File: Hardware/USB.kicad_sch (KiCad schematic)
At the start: 28 parts, among them Q1 MBT3904DW1, U3 CH340C, U9 USB251xB, Y1 24MHz

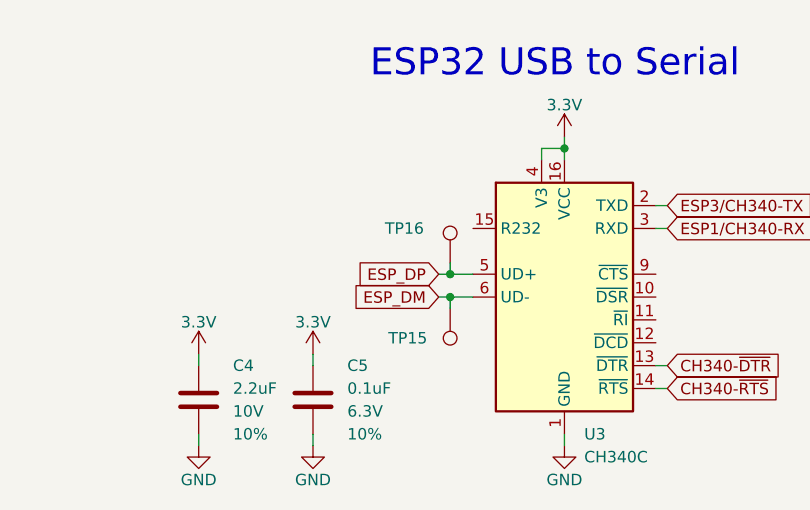
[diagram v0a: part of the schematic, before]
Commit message: Work in progress...
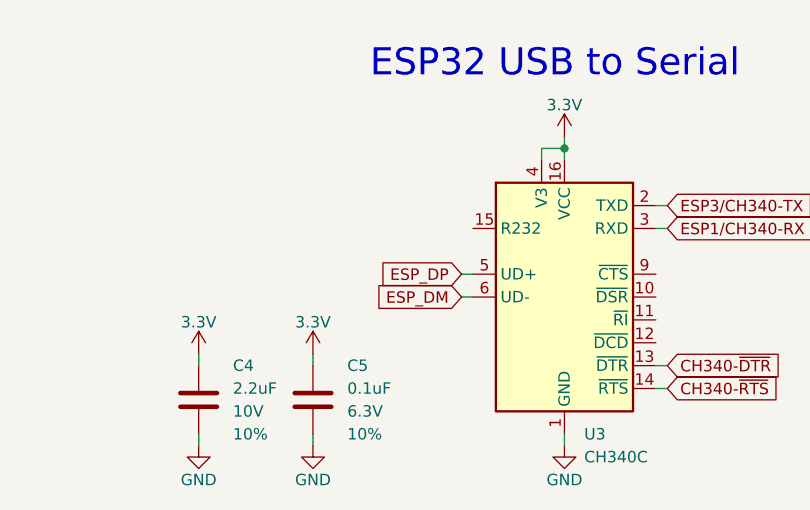
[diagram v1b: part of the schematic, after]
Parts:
- removed TP15, TP16: PTH, SparkFun-Connector:1X01, symbol SparkFun-Connector:TestPoint_PTH
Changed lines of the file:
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@@
   (junction (at 93.98 45.72) (diameter 0) (color 0 0 0 0)
   )
-  (junction (at 110.49 129.54) (diameter 0) (color 0 0 0 0)
-  )
   (junction (at 173.99 139.7) (diameter 0) (color 0 0 0 0)
   )
@@
   (junction (at 162.56 73.66) (diameter 0) (color 0 0 0 0)
   )
-  (junction (at 110.49 127) (diameter 0) (color 0 0 0 0)
-  )
   (junction (at 123.19 113.03) (diameter 0) (color 0 0 0 0)
   )
@@
     (stroke (width 0) (type default))
   )
-  (wire (pts (xy 110.49 125.73) (xy 110.49 127))
-    (stroke (width 0) (type default))
-  )
   (wire (pts (xy 182.88 38.1) (xy 116.84 38.1))
     (stroke (width 0) (type default))
@@
     (stroke (width 0) (type default))
   )
-  (wire (pts (xy 110.49 129.54) (xy 113.03 129.54))
-    (stroke (width 0) (type default))
-  )
   (wire (pts (xy 82.55 137.16) (xy 82.55 135.89))
     (stroke (width 0) (type default))
@@
     (stroke (width 0) (type default))
   )
-  (wire (pts (xy 109.22 127) (xy 110.49 127))
-    (stroke (width 0) (type default))
-  )
   (wire (pts (xy 181.61 78.74) (xy 181.61 80.01))
     (stroke (width 0) (type default))
@@
     (stroke (width 0) (type default))
   )
-  (wire (pts (xy 109.22 129.54) (xy 110.49 129.54))
+  (wire (pts (xy 111.76 129.54) (xy 113.03 129.54))
     (stroke (width 0) (type default))
   )
@@
     (stroke (width 0) (type default))
   )
-  (wire (pts (xy 110.49 129.54) (xy 110.49 130.81))
-    (stroke (width 0) (type default))
-  )
-  (wire (pts (xy 110.49 127) (xy 113.03 127))
+  (wire (pts (xy 111.76 127) (xy 113.03 127))
     (stroke (width 0) (type default))
   )
@@
     )
   )
-  (global_label "ESP_DM" (shape input) (at 109.22 129.54 180) (fields_autoplaced)
+  (global_label "ESP_DM" (shape input) (at 111.76 129.54 180) (fields_autoplaced)
     (effects (font (size 1.27 1.27)) (justify right))
-    (property "Intersheetrefs" "${INTERSHEET_REFS}" (at 98.9173 129.54 0)
+    (property "Intersheetrefs" "${INTERSHEET_REFS}" (at 101.4573 129.54 0)
       (effects (font (size 1.27 1.27)) (justify right) hide)
     )
   )
-  (global_label "ESP_DP" (shape input) (at 109.22 127 180) (fields_autoplaced)
+  (global_label "ESP_DP" (shape input) (at 111.76 127 180) (fields_autoplaced)
     (effects (font (size 1.27 1.27)) (justify right))
-    (property "Intersheetrefs" "${INTERSHEET_REFS}" (at 99.0987 127 0)
+    (property "Intersheetrefs" "${INTERSHEET_REFS}" (at 101.6387 127 0)
       (effects (font (size 1.27 1.27)) (justify right) hide)
     )
@@
         (path "/e3dd3ae4-244d-4cba-9cca-5d2abf83f29a/0cda3e5b-c4bb-4a16-94d7-679fa3b0b0b8"
           (reference "C5") (unit 1)
-        )
-      )
-    )
-  )
-  (symbol (lib_id "SparkFun-Connector:TestPoint_PTH") (at 110.49 130.81 180) (unit 1)
-    (in_bom yes) (on_board yes) (dnp no) (fields_autoplaced)
-    (property "Reference" "TP15" (at 107.95 134.112 0)
-      (effects (font (size 1.27 1.27)) (justify left))
-    )
-    (property "Value" "PTH" (at 110.49 127 0)
-      (effects (font (size 1.27 1.27)) hide)
-    )
-    (property "Footprint" "SparkFun-Connector:1X01" (at 111.76 124.46 0)
-      (effects (font (size 1.27 1.27)) hide)
-    )
-    (property "Datasheet" "~" (at 110.49 123.19 0)
-      (effects (font (size 1.27 1.27)) hide)
-    )
-    (pin "1")
-    (instances
-      (project "SparkFun_RTK_Facet_mosaic"
-        (path "/e3dd3ae4-244d-4cba-9cca-5d2abf83f29a/0cda3e5b-c4bb-4a16-94d7-679fa3b0b0b8"
-          (reference "TP15") (unit 1)
         )
       )
@@
         )
       )
-    )
-  )
-  (symbol (lib_id "SparkFun-Connector:TestPoint_PTH") (at 110.49 125.73 0) (unit 1)
-    (in_bom yes) (on_board yes) (dnp no)
-    (property "Reference" "TP16" (at 105.41 121.92 0)
-      (effects (font (size 1.27 1.27)))
-    )
-    (property "Value" "PTH" (at 110.49 129.54 0)
-      (effects (font (size 1.27 1.27)) hide)
-    )
-    (property "Footprint" "SparkFun-Connector:1X01" (at 109.22 132.08 0)
-      (effects (font (size 1.27 1.27)) hide)
-    )
-    (property "Datasheet" "~" (at 110.49 133.35 0)
-      (effects (font (size 1.27 1.27)) hide)
-    )
-    (pin "1")
-    (instances
-      (project "SparkFun_RTK_Facet_mosaic"
-        (path "/e3dd3ae4-244d-4cba-9cca-5d2abf83f29a/0cda3e5b-c4bb-4a16-94d7-679fa3b0b0b8"
-          (reference "TP16") (unit 1)
-        )
-      )

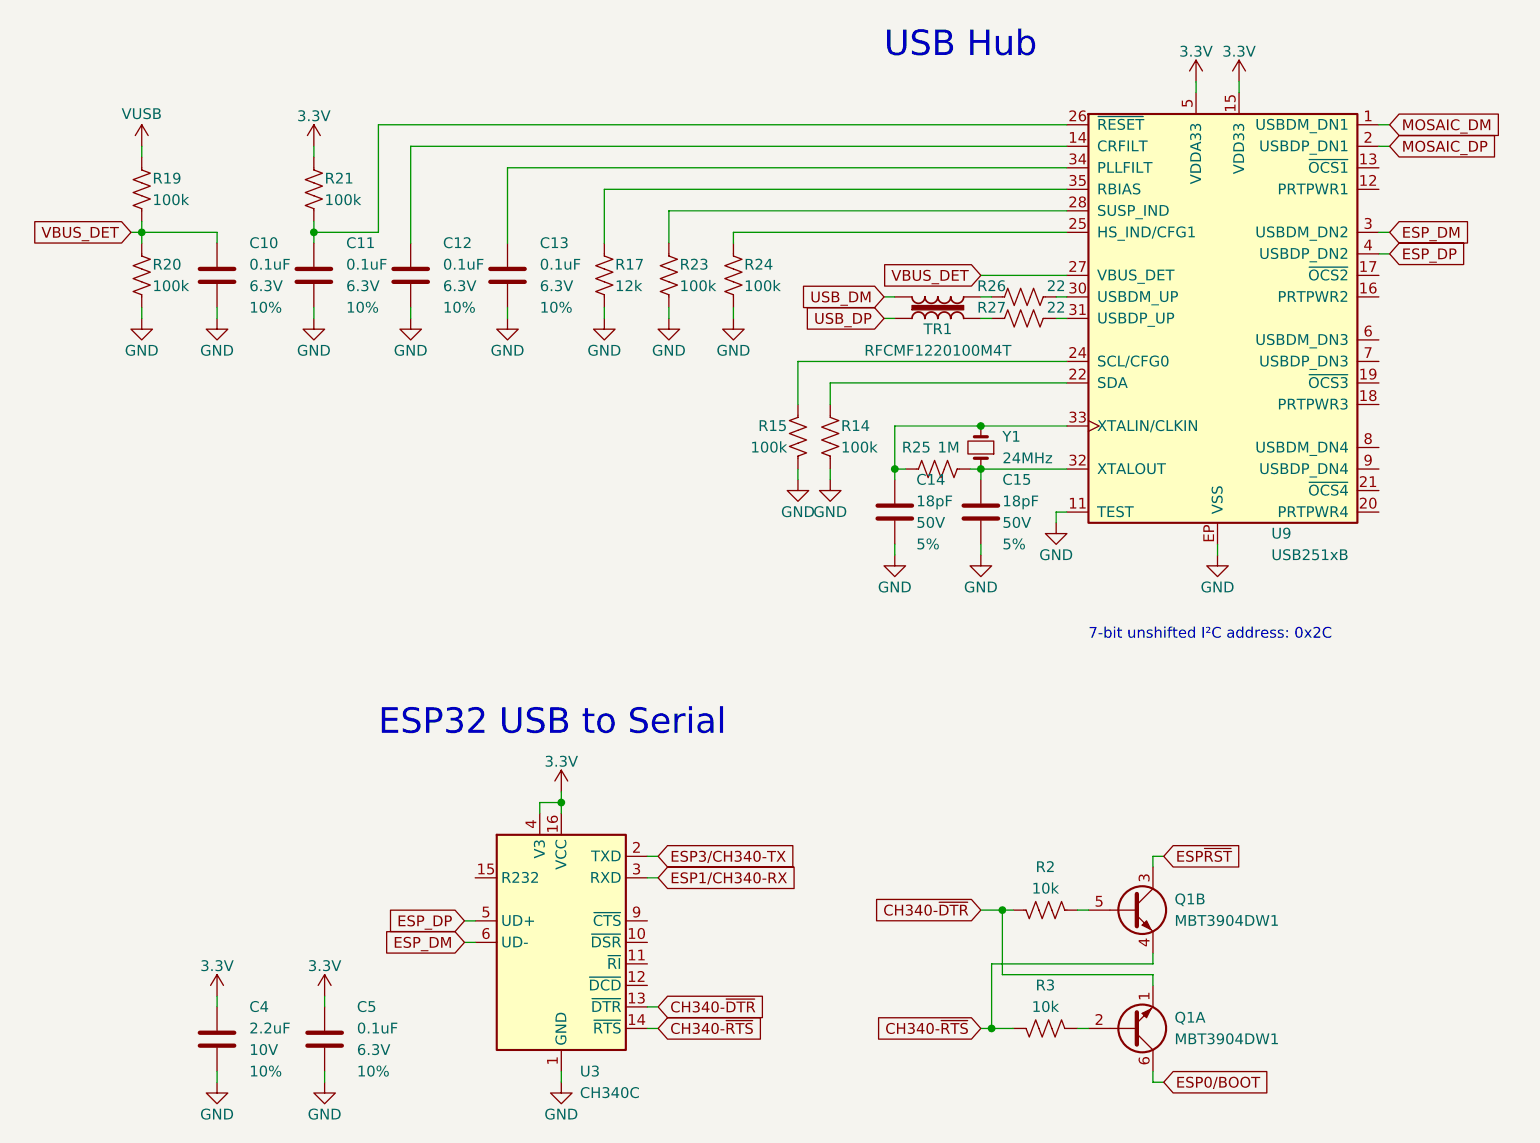
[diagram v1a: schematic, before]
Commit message: Routed
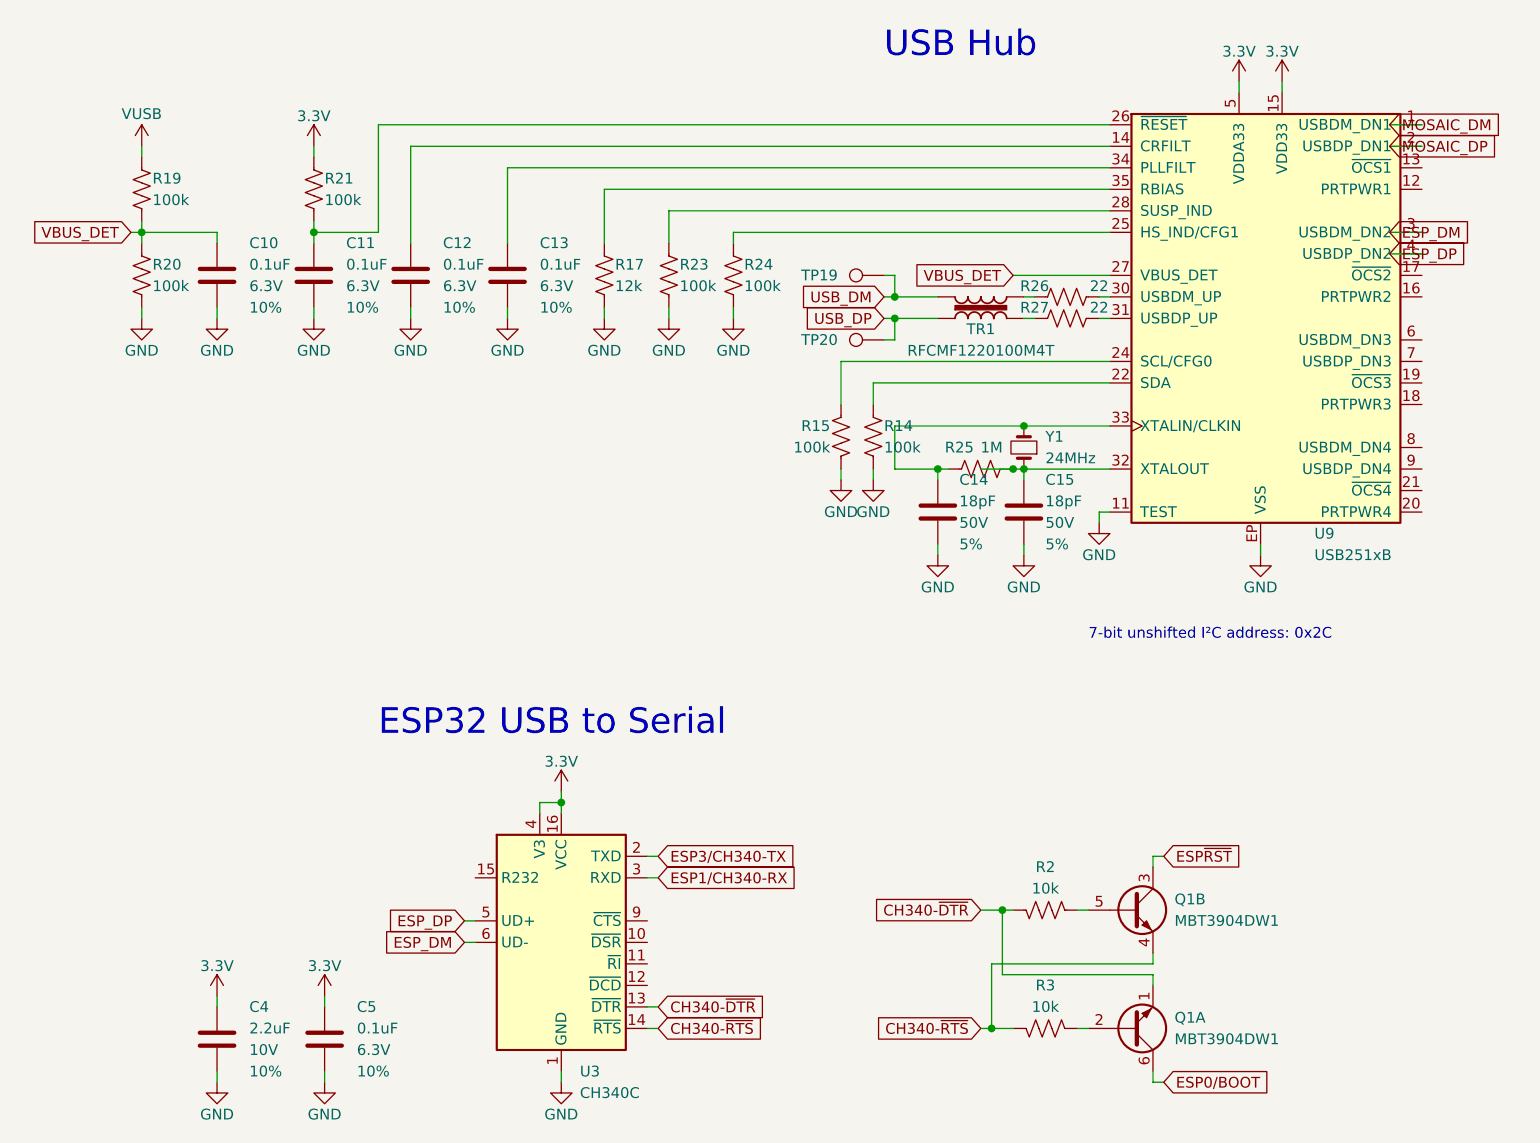
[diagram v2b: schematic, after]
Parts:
- added TP19, TP20: 1.0mm, SparkFun-Connector:TestPoint-1.0mm, symbol SparkFun-Connector:TestPoint_1.0mm
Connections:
- net USB_DM: now also TP19.1
- net USB_DP: now also TP20.1
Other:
- moved on the sheet: C14, C15, R14, R15, R25, R26, R27, TR1, U9, Y1
